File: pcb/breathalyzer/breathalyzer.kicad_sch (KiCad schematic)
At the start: 17 parts, among them IC1 TPS3840DL25DBVR, U1 STM32F030K6Tx, U2 TLV73325PDBV, U3 TLV61070ADBV

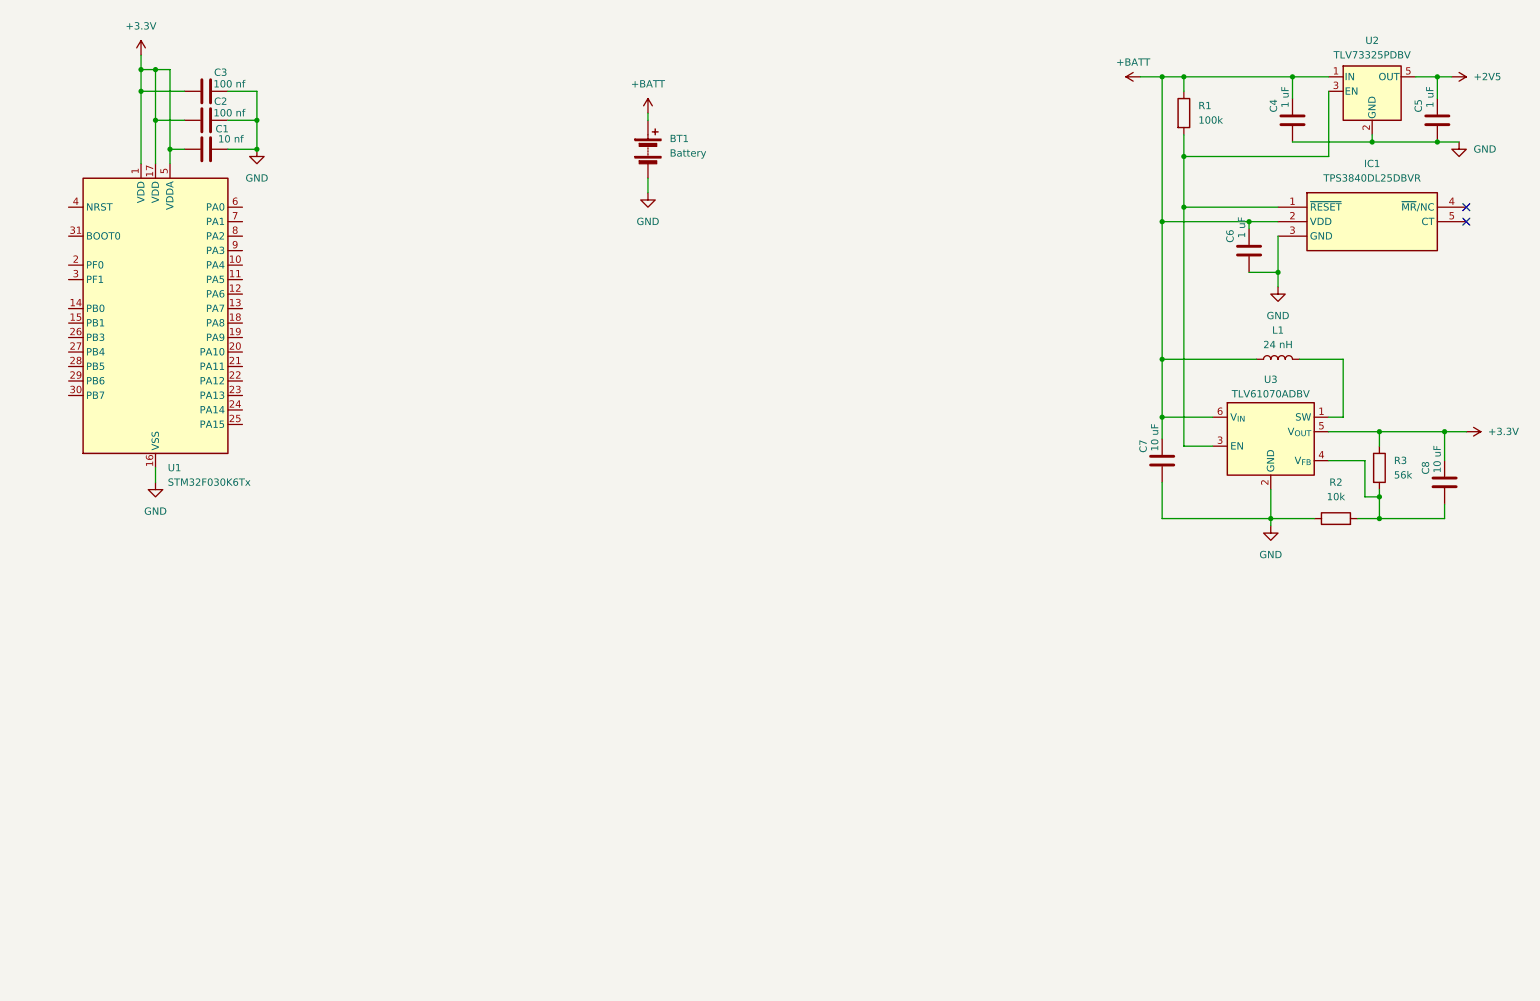
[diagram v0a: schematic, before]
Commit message: program MCU
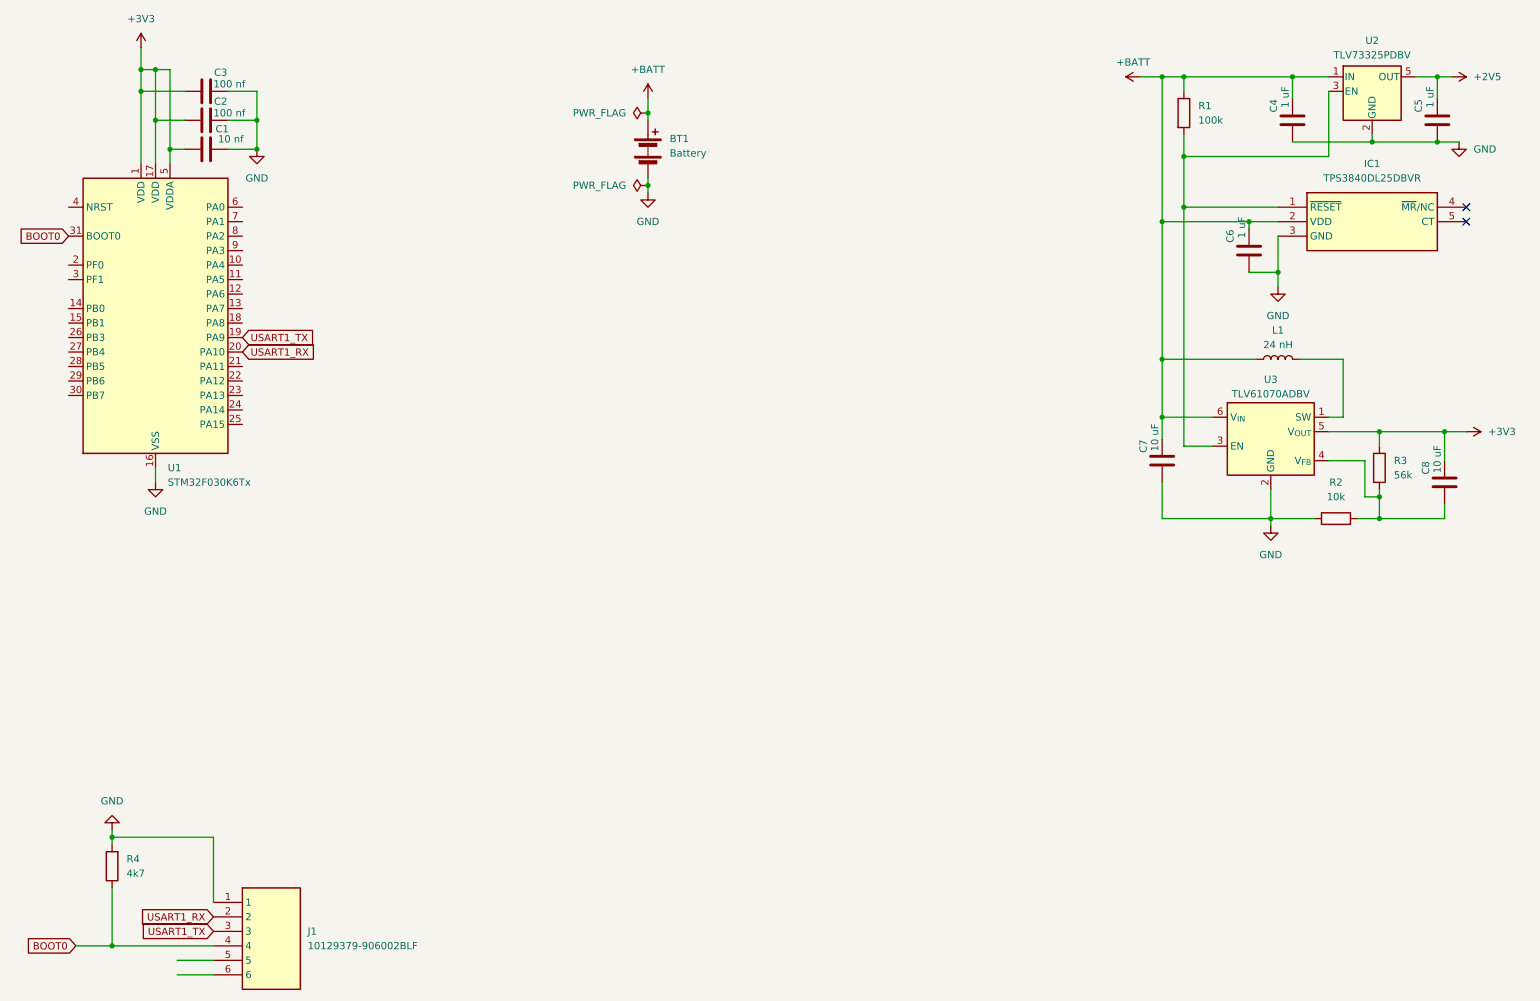
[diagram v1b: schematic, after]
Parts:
- added J1: 10129379-906002BLF, HDRRA6W67P0X254_1X6_1524X254X241P, symbol breathalyzer:10129379-906002BLF
- added R4: 4k7, Resistor_SMD:R_1206_3216Metric, symbol Device:R
- IC1: footprint SOT95P280X145-5N -> Package_TO_SOT_SMD:SOT-23-5_HandSoldering
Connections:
- net GND: now also J1.1, R4.2
- net USART1_TX: now reaches U1.19 (PA9)
- net USART1_TX: now also J1.3
- net USART1_RX: now reaches U1.20 (PA10)
- net USART1_RX: now also J1.2
- net BOOT0: now reaches U1.31 (BOOT0)
- net BOOT0: now also J1.4, R4.1
- net +3.3V renamed +3V3

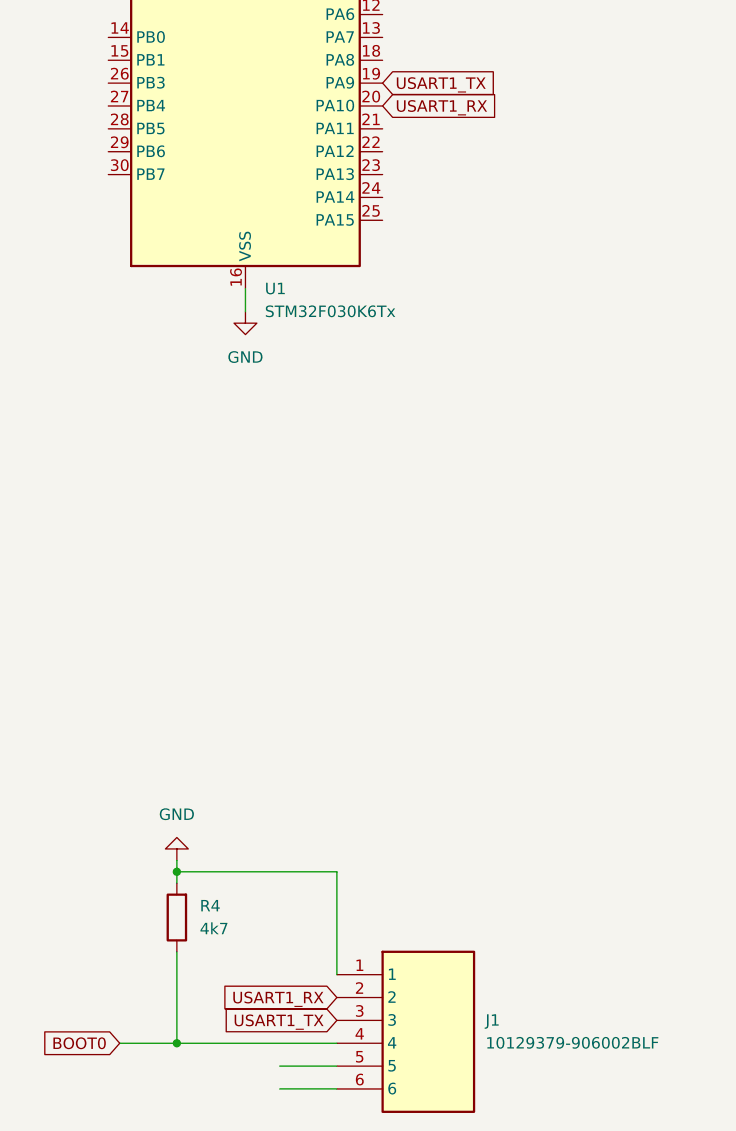
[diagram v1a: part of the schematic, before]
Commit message: Serial debug
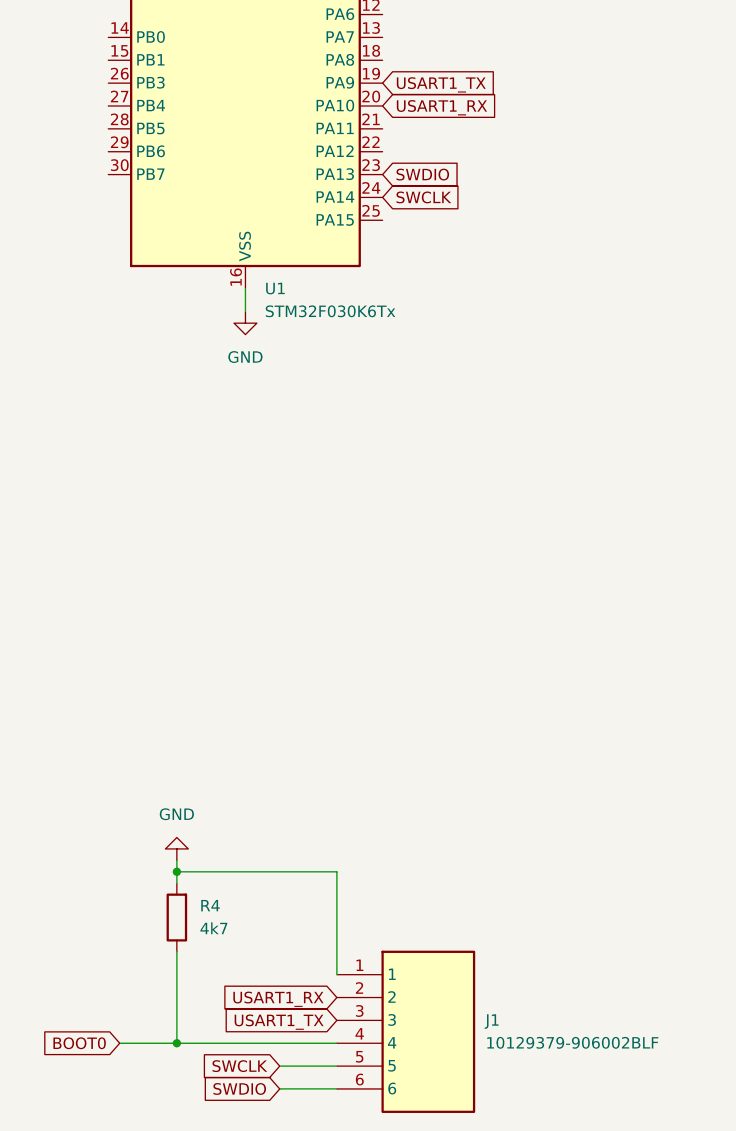
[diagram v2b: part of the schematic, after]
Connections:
- net SWCLK: now reaches J1.5
- net SWCLK: now also U1.24 (PA14)
- net SWDIO: now reaches J1.6
- net SWDIO: now also U1.23 (PA13)
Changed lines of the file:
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@@
+		)
+	)
+	(global_label "SWDIO"
+		(shape input)
+		(at 59.69 80.01 0)
+		(fields_autoplaced yes)
+		(effects
+			(font
+				(size 1.27 1.27)
+			)
+			(justify left)
+		)
+		(property "Intersheetrefs" "${INTERSHEET_REFS}"
+			(at 68.5414 80.01 0)
+			(effects
+				(font
+					(size 1.27 1.27)
+				)
+				(justify left)
+				(hide yes)
+			)
 		)
 	)
@@
 				)
 				(justify left)
+				(hide yes)
+			)
+		)
+	)
+	(global_label "SWCLK"
+		(shape input)
+		(at 59.69 82.55 0)
+		(fields_autoplaced yes)
+		(effects
+			(font
+				(size 1.27 1.27)
+			)
+			(justify left)
+		)
+		(property "Intersheetrefs" "${INTERSHEET_REFS}"
+			(at 68.9042 82.55 0)
+			(effects
+				(font
+					(size 1.27 1.27)
+				)
+				(justify left)
+				(hide yes)
+			)
+		)
+	)
+	(global_label "SWDIO"
+		(shape input)
+		(at 48.26 181.61 180)
+		(fields_autoplaced yes)
+		(effects
+			(font
+				(size 1.27 1.27)
+			)
+			(justify right)
+		)
+		(property "Intersheetrefs" "${INTERSHEET_REFS}"
+			(at 39.4086 181.61 0)
+			(effects
+				(font
+					(size 1.27 1.27)
+				)
+				(justify right)
 				(hide yes)
 			)
@@
 				(hide yes)
 			)
+		)
+	)
+	(global_label "SWCLK"
+		(shape input)
+		(at 48.26 179.07 180)
+		(fields_autoplaced yes)
+		(effects
+			(font
+				(size 1.27 1.27)
+			)
+			(justify right)
+		)
+		(property "Intersheetrefs" "${INTERSHEET_REFS}"
+			(at 39.0458 179.07 0)
+			(effects
+				(font
+					(size 1.27 1.27)
+				)
+				(justify right)
+				(hide yes)
+			)
